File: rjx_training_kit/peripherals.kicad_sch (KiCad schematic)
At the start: 39 parts, among them J5 LiPo_4.2V, J6 CR2032_3V, Q1 BC817, Q2 BC817, SW2 SW_Push, U3 BME280, U4 BQ27441-G1, U5 PCF8563T, U6 LIS3DH, Y1 32.768kHz

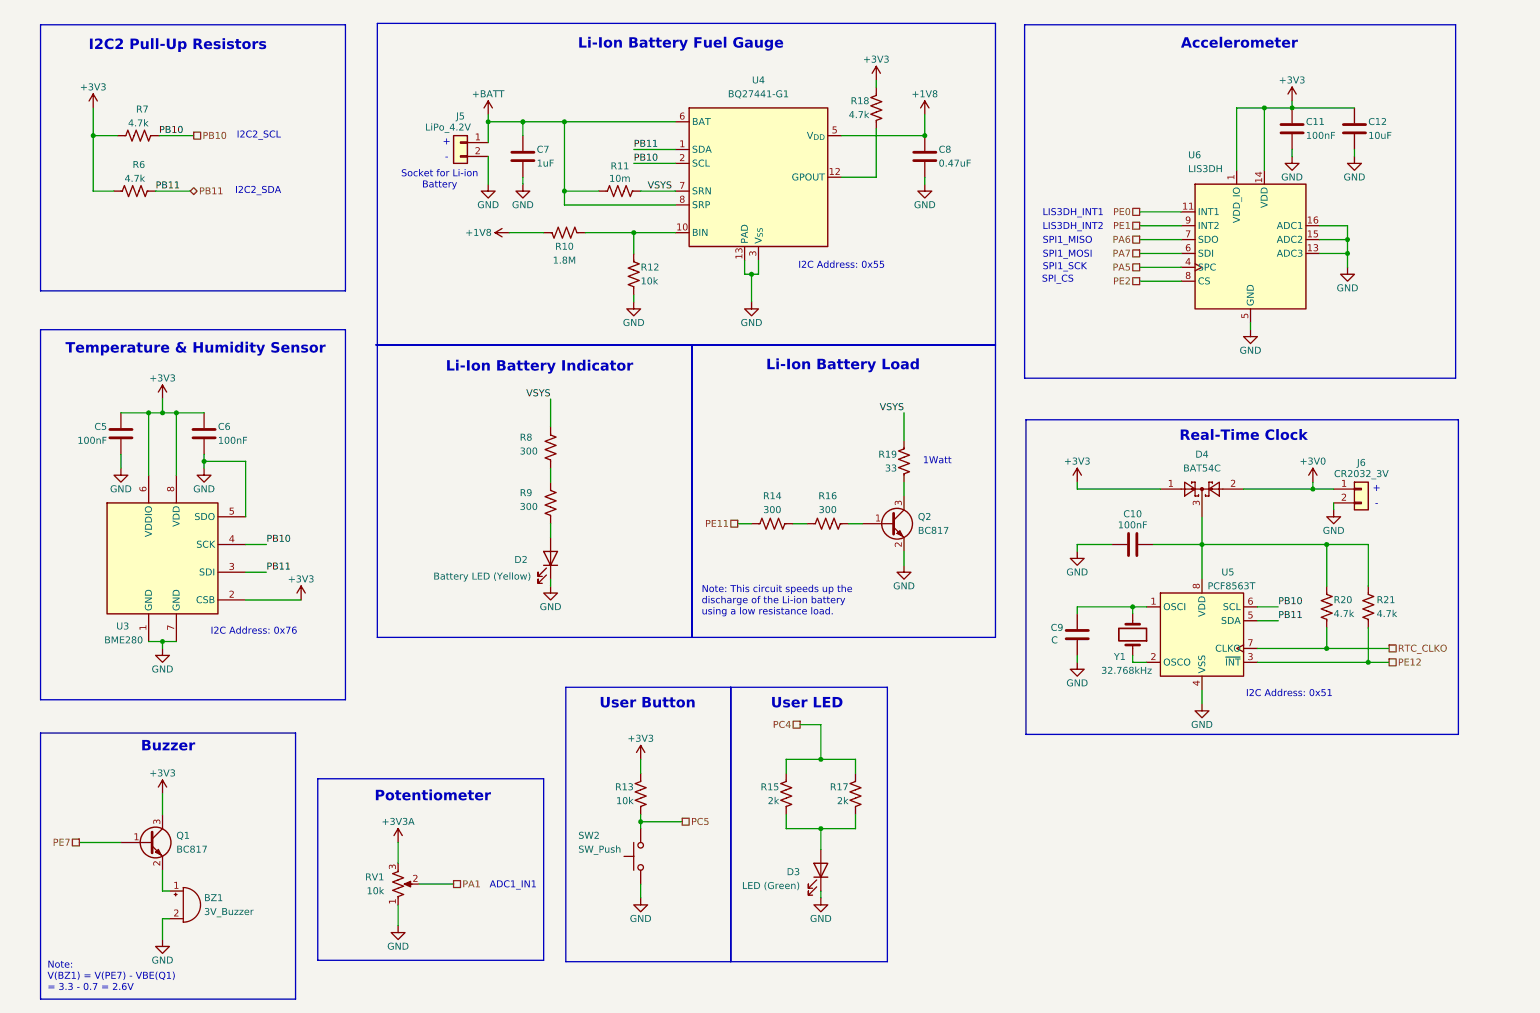
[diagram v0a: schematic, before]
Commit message: Update
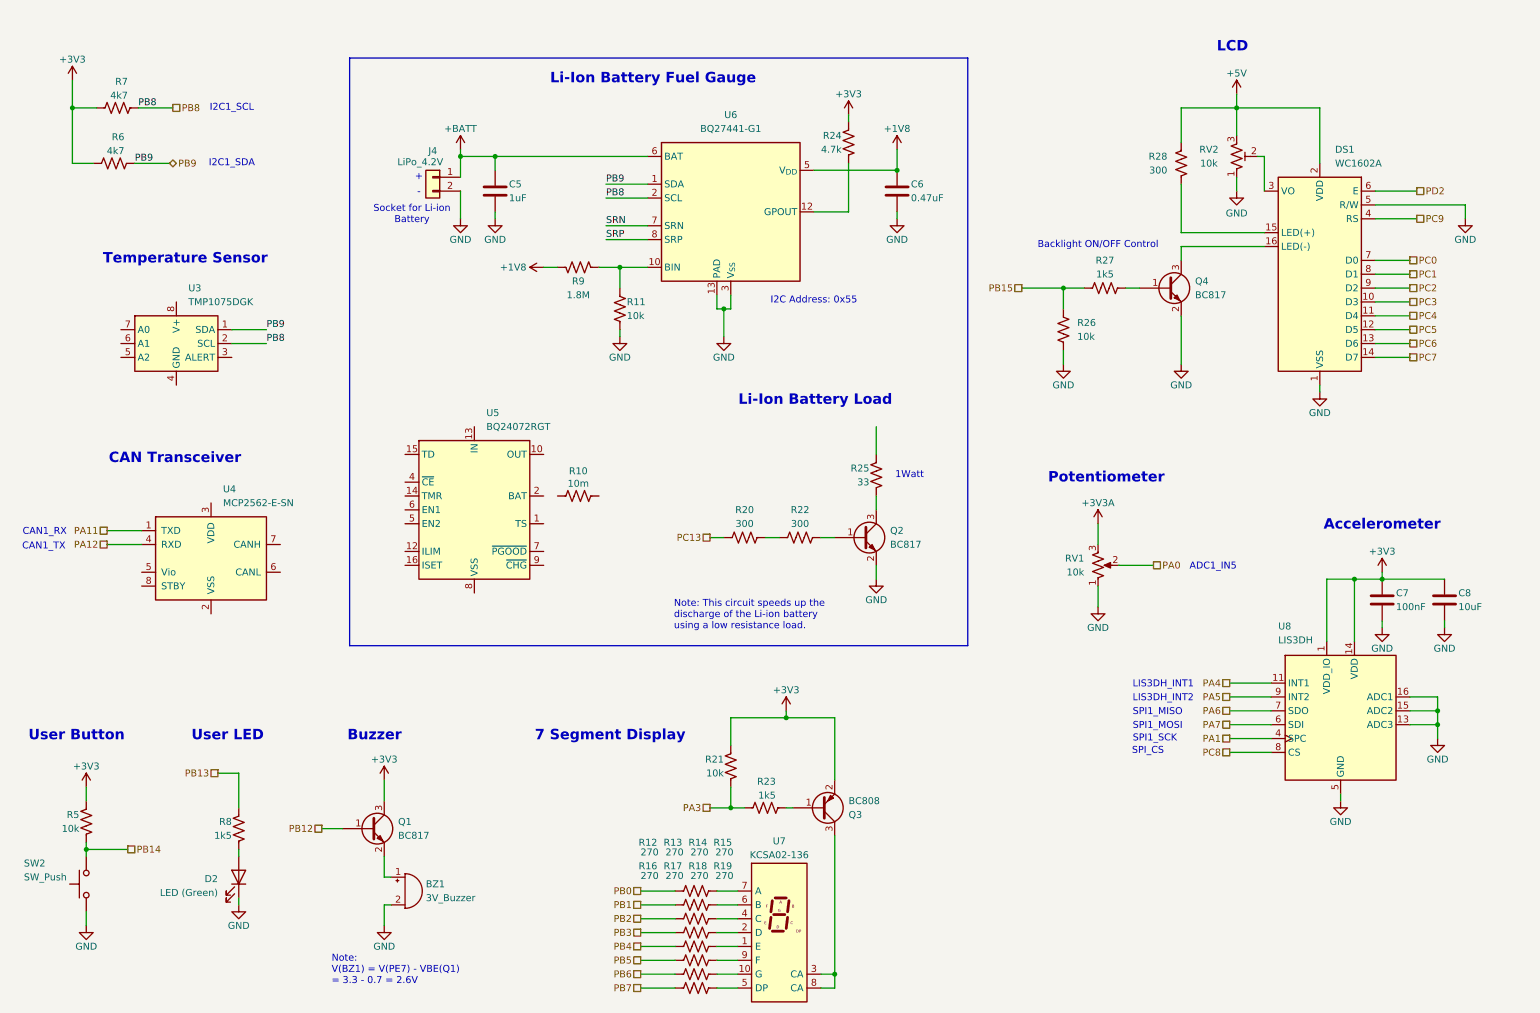
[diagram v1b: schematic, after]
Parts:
- removed C10, C5, C6: 100nF, symbol Device:C
- removed C9: C, symbol Device:C
- removed D2: Battery LED (Yellow), symbol Device:LED
- removed D4: BAT54C, Package_TO_SOT_SMD:SOT-23, symbol Diode:BAT54C
- removed J6: CR2032_3V, symbol Connector_Generic:Conn_01x02
- removed R11: 10m, symbol Device:R_US
- removed R20: 4.7k, symbol Device:R_US
- removed R8, R9: 300, symbol Device:R_US
- removed U3: BME280, Package_LGA:Bosch_LGA-8_2.5x2.5mm_P0.65mm_ClockwisePinNumbering, symbol Sensor:BME280
- removed U5: PCF8563T, Package_SO:SOIC-8_3.9x4.9mm_P1.27mm, symbol Timer_RTC:PCF8563T
- removed Y1: 32.768kHz, symbol Device:Crystal
- added DS1: WC1602A, Display:WC1602A, symbol Display_Character:WC1602A
- added Q3: BC808, Package_TO_SOT_SMD:SOT-23, symbol Transistor_BJT:BC808
- added Q4: BC817, Package_TO_SOT_SMD:SOT-23, symbol Transistor_BJT:BC817
- added R10: 10m, symbol Device:R_US
- added R12, R13, R14, R15, R16, R18, R19: 270, symbol Device:R_US
- added R23, R27: 1k5, symbol Device:R_US
- added R26: 10k, symbol Device:R_US
- added R28: 300, symbol Device:R_US
- added RV2: 10k, symbol Device:R_Potentiometer_Trim_US
- added U3: TMP1075DGK, Package_SO:VSSOP-8_3x3mm_P0.65mm, symbol Sensor_Temperature:TMP1075DGK
- added U4: MCP2562-E-SN, Package_SO:SOIC-8_3.9x4.9mm_P1.27mm, symbol Interface_CAN_LIN:MCP2562-E-SN
- added U5: BQ24072RGT, Package_DFN_QFN:VQFN-16-1EP_3x3mm_P0.5mm_EP1.6x1.6mm, symbol Battery_Management:BQ24072RGT
- added U7: KCSA02-136, Display_7Segment:KCSC02-136, symbol Display_Character:KCSA02-136
- R17: value 2k -> 270
- R21: value 4.7k -> 10k
- R6, R7: value 4.7k -> 4k7
- R8: renamed from R15; value 2k -> 1k5
- renumbered C7 to C5, C8 to C6, C11 to C7, C12 to C8, D3 to D2, J5 to J4, R12 to R11, R14 to R20, R16 to R22, R18 to R24, R19 to R25, R13 to R5, R10 to R9, U4 to U6, U6 to U8
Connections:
- net PE1 is gone; now on net PA5: U8.9 (INT2)
- net +3V3: now also R21.1, Q3.2 (E)
- net +BATT: no longer U6.8 (SRP)
- net GND: now also DS1.1 (VSS), DS1.5 (R/W), Q4.2 (E), R26.2, RV2.1
- net PA1: now also U8.4 (SPC); no longer RV1.2
- net PA5: no longer U8.4 (SPC)
- net PC4: now also DS1.11 (D4); no longer R17.1, R8.1
- net PC5: now also DS1.12 (D5); no longer R5.2, SW2.2
- net at D2.2 (A), R8.2: no longer R17.2
- net PB10 renamed PB8
- net PB8: now also U3.2 (SCL)
- net PB11 renamed PB9
- net PB9: now also U3.1 (SDA)
- net PE0 renamed PA4
- net PE11 renamed PC13
- net PE12 renamed PA3
- net PA3: now also R23.1
- net PE2 renamed PC8
- net PE7 renamed PB12
- net VSYS: no longer names the net of R25.1
- net VSYS: no longer U6.7 (SRN)
- new net: R18.2, U7.10 (G)
- new net: Q4.1 (B), R27.2
- new net: R13.2, U7.6 (B)
- new net: Q3.1 (B), R23.2
- new net: DS1.15 (LED(+)), R28.1
- new net: DS1.16 (LED(-)), Q4.3 (C)
- new net: Q3.3 (C), U7.3 (CA), U7.8 (CA)
- new net: R15.2, U7.2 (D)
- new net: DS1.3 (VO), RV2.2
- new net: R12.2, U7.7 (A)
- new net: R17.2, U7.9 (F)
- new net: R16.2, U7.1 (E)
- new net: R19.2, U7.5 (DP)
- new net: R14.2, U7.4 (C)
- new net: U5.10 (OUT), U5.11 (OUT)
- new net: U5.17 (VSS), U5.8 (VSS)
- new net: U5.2 (BAT), U5.3 (BAT)
- new net +5V: DS1.2 (VDD), R28.2, RV2.3
- new net PA0: RV1.2
- new net PA11: U4.1 (TXD)
- new net PA12: U4.4 (RXD)
- new net PB0: R12.1
- new net PB1: R13.1
- new net PB13: R8.1
- new net PB14: R5.2, SW2.2
- new net PB15: R26.1, R27.1
- new net PB2: R14.1
- new net PB3: R15.1
- new net PB4: R16.1
- new net PB5: R17.1
- new net PB6: R18.1
- new net PB7: R19.1
- new net PC0: DS1.7 (D0)
- new net PC1: DS1.8 (D1)
- new net PC2: DS1.9 (D2)
- new net PC3: DS1.10 (D3)
- new net PC6: DS1.13 (D6)
- new net PC7: DS1.14 (D7)
- new net PC9: DS1.4 (RS)
- new net PD2: DS1.6 (E)
- new net SRN: U6.7 (SRN)
- new net SRP: U6.8 (SRP)
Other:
- note added: "7 Segment Display"
- note added: "ADC1_IN5"
- note added: "Backlight ON/OFF Control"
- note added: "CAN Transceiver"
- note added: "CAN1_RX"
- note added: "CAN1_TX"
- note added: "I2C1_SCL"
- note added: "I2C1_SDA"
- note added: "LCD"
- note added: "Temperature Sensor"
- note removed: "ADC1_IN1"
- note removed: "I2C Address: 0x51"
- note removed: "I2C Address: 0x76"
- note removed: "I2C2 Pull-Up Resistors"
- note removed: "I2C2_SCL"
- note removed: "I2C2_SDA"
- note removed: "Li-Ion Battery Indicator"
- note removed: "Real-Time Clock"
- note removed: "Temperature & Humidity Sensor"
- moved on the sheet: BZ1, C5, C6, C7, C8, D2, J4, Q1, Q2, R11, R20, R22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

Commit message: Update
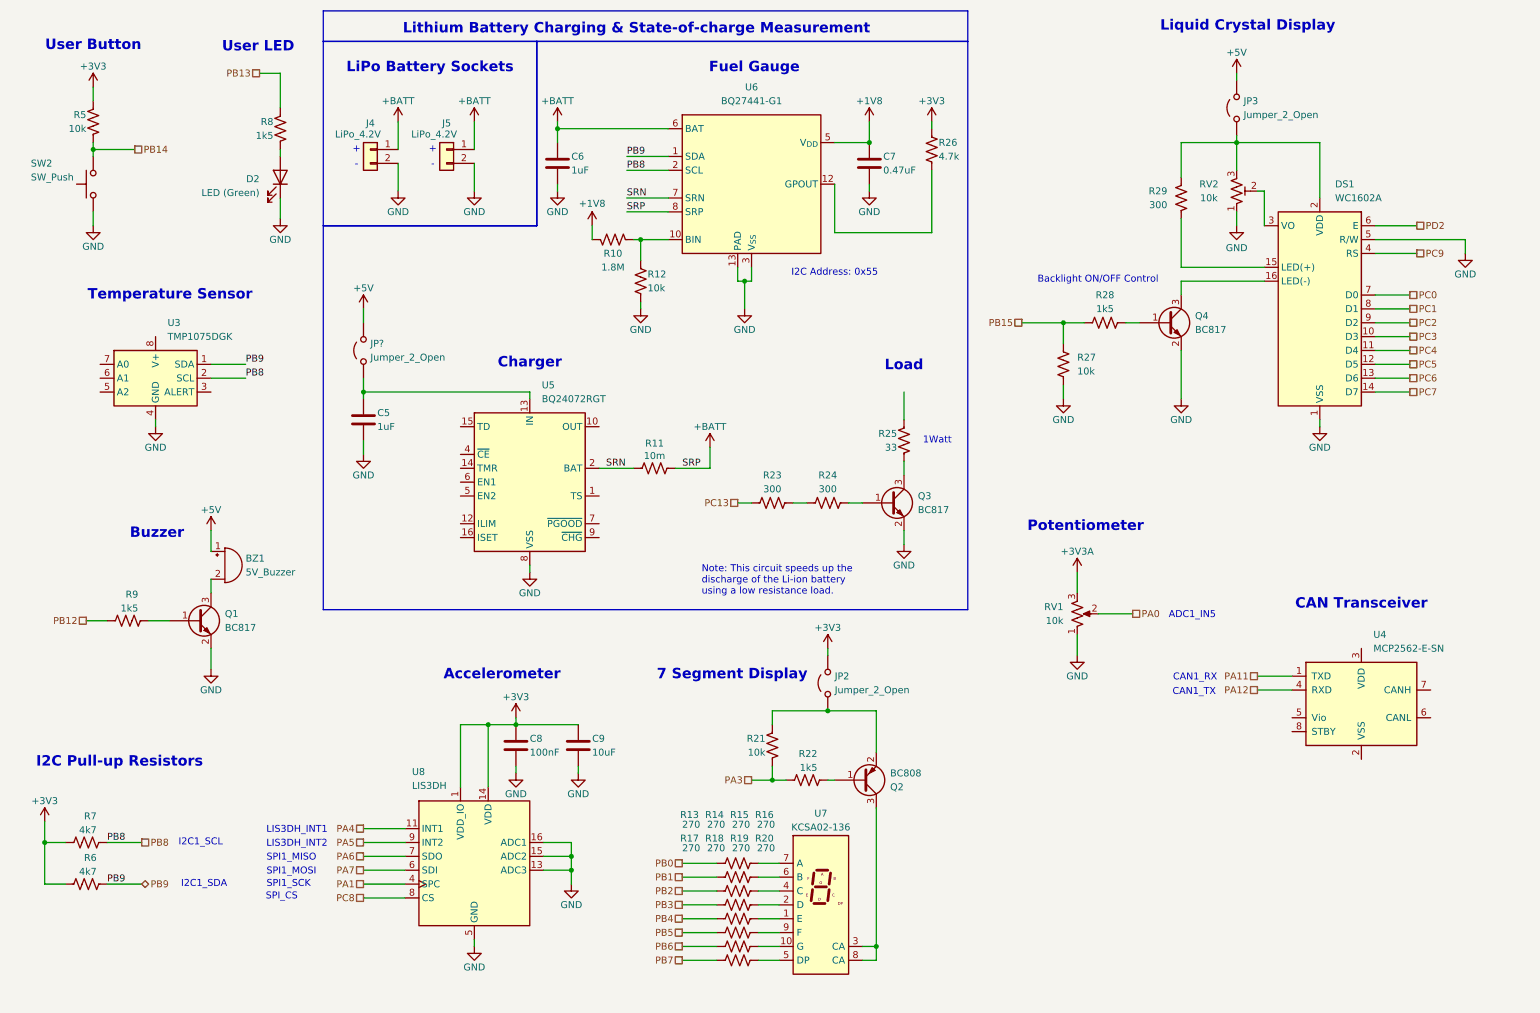
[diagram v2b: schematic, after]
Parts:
- added C5: 1uF, symbol Device:C
- added J5: LiPo_4.2V, symbol Connector_Generic:Conn_01x02
- added JP2, JP3, JP?: Jumper_2_Open, symbol Jumper:Jumper_2_Open
- added R9: 1k5, symbol Device:R_US
- BZ1: value 3V_Buzzer -> 5V_Buzzer
- renumbered C5 to C6, C6 to C7, C7 to C8, C8 to C9, Q3 to Q2, Q2 to Q3, R9 to R10, R10 to R11, R11 to R12, R12 to R13, R13 to R14, R14 to R15, R15 to R16, R16 to R17, R17 to R18, R18 to R19, R19 to R20, R23 to R22, R20 to R23, R22 to R24, R24 to R26, R26 to R27, R27 to R28, R28 to R29
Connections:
- net SRP is gone; now on net +BATT: U6.8 (SRP)
- net +3V3: now also JP2.2 (B); no longer Q1.3 (C), Q2.2 (E), R21.1
- net +5V: now also BZ1.1 (+), JP3.2 (B), JP?.2 (B); no longer DS1.2 (VDD), R29.2, RV2.3
- net +BATT: now also R11.2, J5.1 (Pin_1)
- net GND: now also Q1.2 (E), U3.4 (GND), U5.17 (VSS), U5.8 (VSS), C5.2, J5.2 (Pin_2); no longer BZ1.2 (-)
- net PB12: now also R9.1; no longer Q1.1 (B)
- net SRN: now also R11.1, U5.2 (BAT), U5.3 (BAT)
- net at U5.13 (IN): now also C5.1, JP?.1 (A)
- new net: JP2.1 (A), Q2.2 (E), R21.1
- new net: Q1.1 (B), R9.2
- new net: DS1.2 (VDD), JP3.1 (A), R29.2, RV2.3
- new net: BZ1.2 (-), Q1.3 (C)
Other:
- note added: "Charger"
- note added: "Fuel Gauge"
- note added: "I2C Pull-up Resistors"
- note added: "LiPo Battery Sockets"
- note added: "Liquid Crystal Display"
- note added: "Lithium Battery Charging & State-of-charge Measurement"
- note added: "Load"
- note removed: "LCD"
- note removed: "Li-Ion Battery Fuel Gauge"
- note removed: "Li-Ion Battery Load"
- note removed: "Note: V(BZ1) = V(PE7) - VBE(Q1) = 3.3 - 0.7 = 2.6V"
- note removed: "Socket for Li-ion Battery"
- moved on the sheet: BZ1, C6, C7, C8, C9, D2, DS1, J4, Q1, Q2, Q3, Q4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
